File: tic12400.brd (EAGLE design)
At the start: 100 x 80 mm, 58 parts, among them IC1 7805TV, Q1 CSTCR6M00G53Z, U1 TIC12400DCPR, U2 MCZ33996EK, U3 MCP2210-I/SO, U4 BMX160, X1 22-23-2031, X2 INPUT1, X3 INPUT2, X4 INPUT3, X5 22-23-2031, X6 OUTPUT1, X7 OUTPUT2, X8 MINI-USB-32005-201

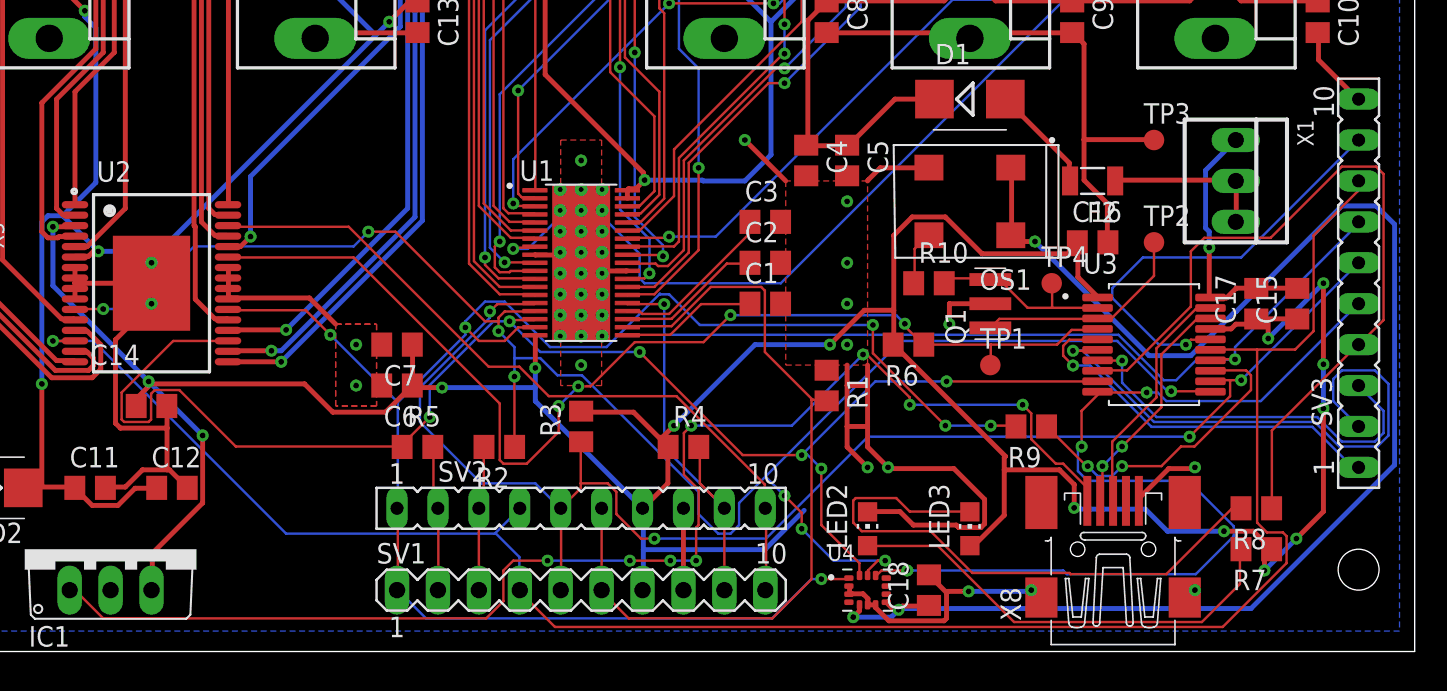
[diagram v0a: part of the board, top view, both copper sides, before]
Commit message: up
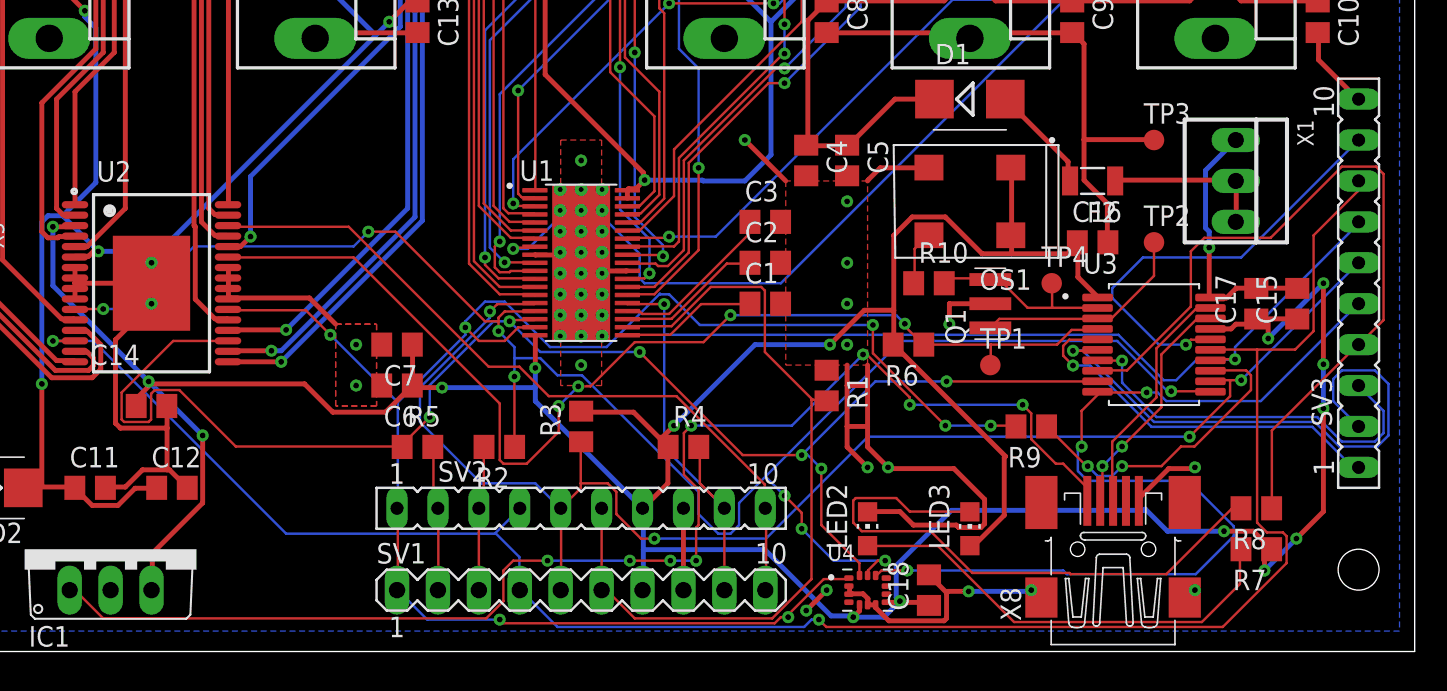
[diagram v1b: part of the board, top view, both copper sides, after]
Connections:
- removed net N$52: C18.1, OS1.1, OS1.4, U4.5, U4.8
- net VDD: now also C18.1, OS1.1, OS1.4, U4.5, U4.8
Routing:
- net N$52: track 91.8 -> 0.00 mm, vias 3 -> 0
- net VDD: track 212.0 -> 236.3 mm, vias 15 -> 16
- net GND: track 174.1 -> 175.9 mm, vias 19 -> 21
- net MISO_JP4P1: track 108.0 -> 108.3 mm, vias 6 -> 7
- net N$65: track 122.4 -> 122.7 mm, vias 1 -> 2
